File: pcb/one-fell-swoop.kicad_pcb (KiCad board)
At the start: 2 copper layers, 107.2 x 86.9 mm, 21 parts, among them J1 MJ-4PP-9, SW1 SW_PUSH, SW10 SW_PUSH, SW11 SW_PUSH, SW12 SW_PUSH, SW13 SW_PUSH, SW14 SW_PUSH, SW15 SW_PUSH, SW16 SW_PUSH, SW17 SW_PUSH, SW2 SW_PUSH, SW3 SW_PUSH, SW4 SW_PUSH, SW5 SW_PUSH, SW6 SW_PUSH, SW7 SW_PUSH, SW8 SW_PUSH, SW9 SW_PUSH, U1 ProMicro

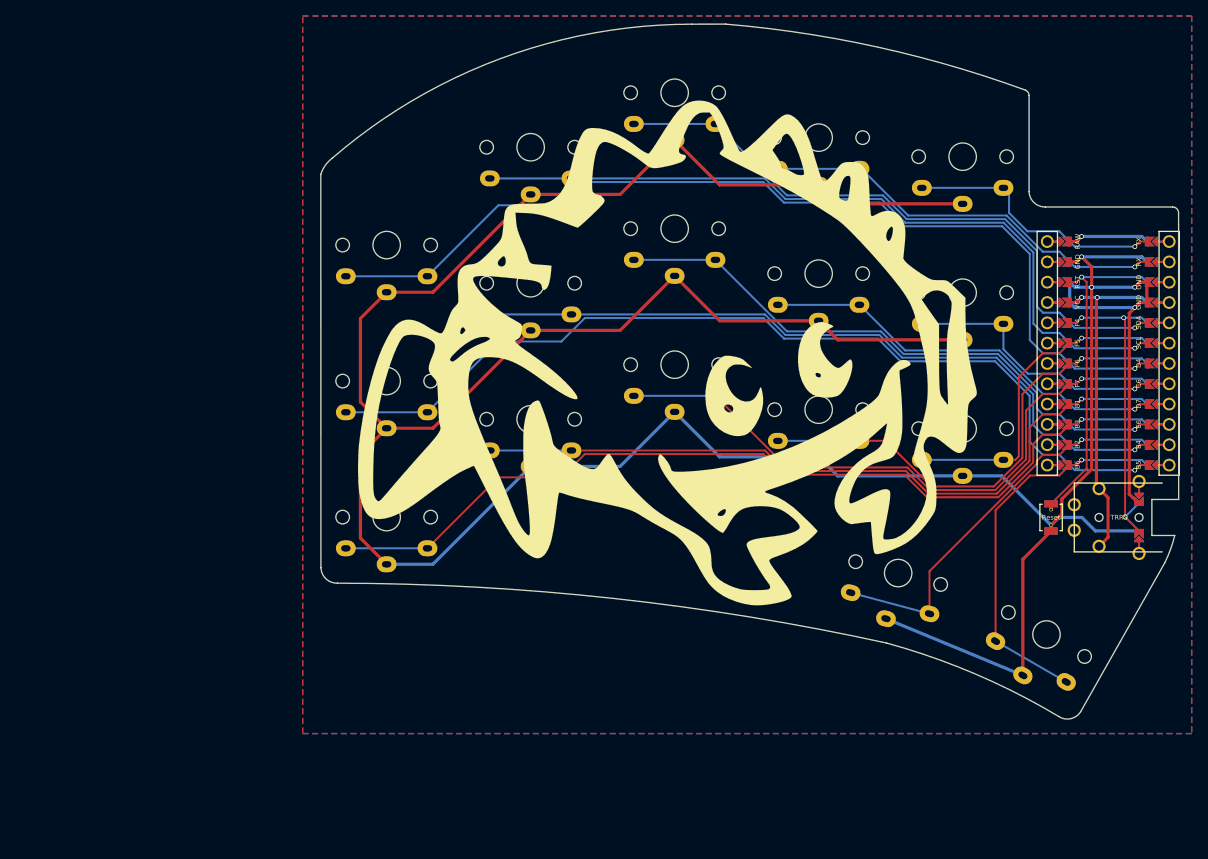
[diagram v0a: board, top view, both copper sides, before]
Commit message: Added files for the second version of the Swoop.
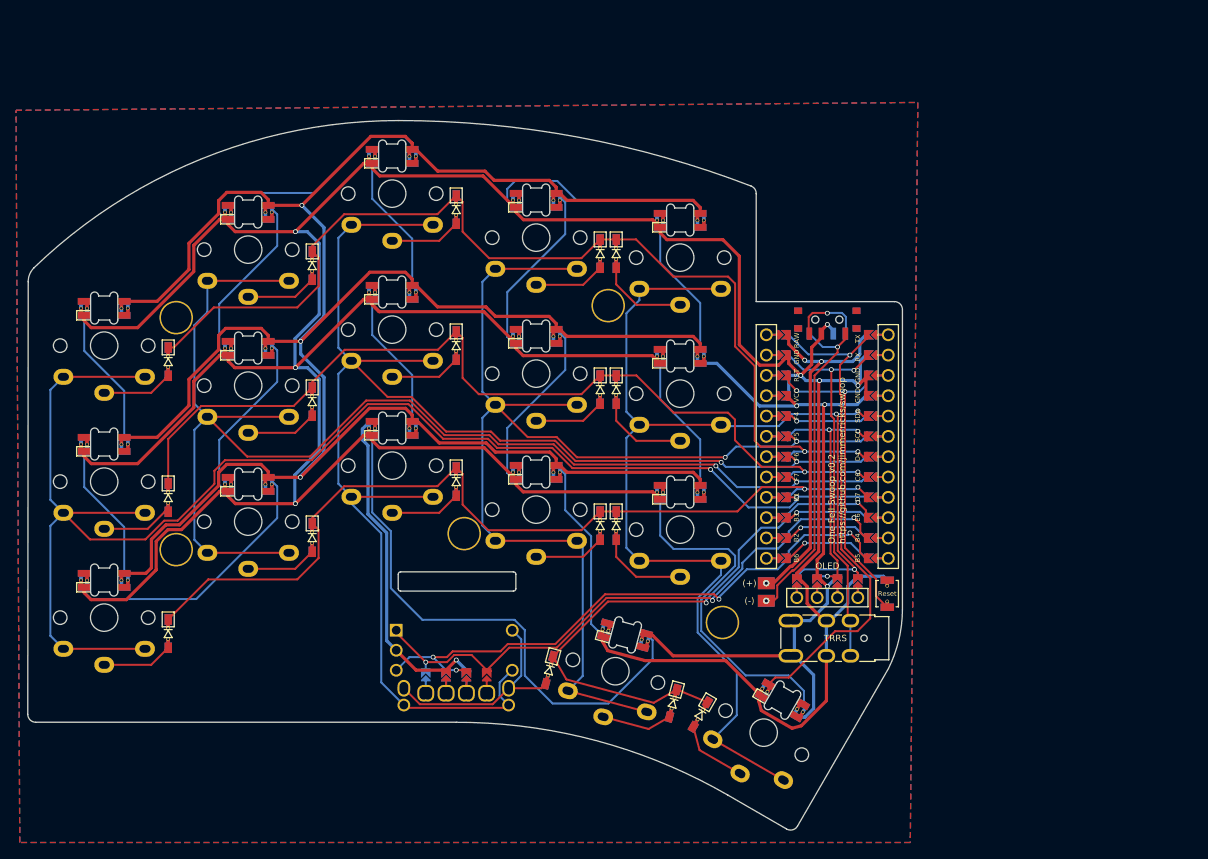
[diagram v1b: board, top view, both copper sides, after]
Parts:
- removed G***: LOGO, one-fell-swoop:Ferris_rust_logos
- added BT1: Battery, swoop:Battery_pads, F.Cu at (154.0, 118.0)
- added D1: 1N4148W, swoop:D3_SMD, F.Cu at (79.2, 89.2)
- added D10: 1N4148W, swoop:D3_SMD, F.Cu at (135.2, 92.7)
- added D11: 1N4148W, swoop:D3_SMD, F.Cu at (79.2, 123.2)
- added D12: 1N4148W, swoop:D3_SMD, F.Cu at (97.2, 111.2)
- added D13: 1N4148W, swoop:D3_SMD, F.Cu at (115.2, 104.2)
- added D14: 1N4148W, swoop:D3_SMD, F.Cu at (133.2, 109.7)
- added D15: 1N4148W, swoop:D3_SMD, F.Cu at (135.2, 109.7)
- added D16: 1N4148W, swoop:D3_SMD, F.Cu at (142.3, 131.9)
- added D17: 1N4148W, swoop:D3_SMD, F.Cu at (145.8, 133.4)
- added D2: 1N4148W, swoop:D3_SMD, F.Cu at (97.2, 77.2)
- added D3: 1N4148W, swoop:D3_SMD, F.Cu at (115.2, 70.2)
- added D4: 1N4148W, swoop:D3_SMD, F.Cu at (133.2, 75.7)
- added D5: 1N4148W, swoop:D3_SMD, F.Cu at (135.2, 75.7)
- added D6: 1N4148W, swoop:D3_SMD, F.Cu at (79.2, 106.2)
- added D7: 1N4148W, swoop:D3_SMD, F.Cu at (97.2, 94.2)
- added D8: 1N4148W, swoop:D3_SMD, F.Cu at (115.2, 87.2)
- added D9: 1N4148W, swoop:D3_SMD, F.Cu at (133.2, 92.7)
- added ED1: 1N4148W, swoop:D3_SMD, F.Cu at (126.9, 127.8)
- added EN1: RotaryEncoder_Switch, swoop:RotaryEncoder, F.Cu at (115.2, 125.3)
- added EN2: EVQWGD001, swoop:RollerEncoder, F.Cu at (115.2, 125.3)
- added H1: M2 Hole, swoop:M2_hole_4.2mm, F.Cu at (80.2, 83.7)
- added H2: M2 Hole, swoop:M2_hole_4.2mm, F.Cu at (80.2, 112.7)
- added H3: M2 Hole, swoop:M2_hole_4.2mm, F.Cu at (134.2, 82.2)
- added H4: M2 Hole, swoop:M2_hole_4.2mm, F.Cu at (116.2, 110.7)
- added H4: M2 Hole, swoop:M2_hole_4.2mm, F.Cu at (148.5, 121.9)
- added L1: SK6812Mini-e, swoop:SK6812_Mini_E, F.Cu at (71.2, 82.7)
- added L10: SK6812Mini-e, swoop:SK6812_Mini_E, F.Cu at (143.2, 88.7)
- added L11: SK6812Mini-e, swoop:SK6812_Mini_E, F.Cu at (71.2, 116.7)
- added L12: SK6812Mini-e, swoop:SK6812_Mini_E, F.Cu at (89.2, 104.7)
- added L13: SK6812Mini-e, swoop:SK6812_Mini_E, F.Cu at (107.2, 97.7)
- added L14: SK6812Mini-e, jmnw:sk6812_mini_e_rev, F.Cu at (125.2, 103.2)
- added L15: SK6812Mini-e, swoop:SK6812_Mini_E, F.Cu at (143.2, 105.7)
- added L16: SK6812Mini-e, swoop:SK6812_Mini_E, F.Cu at (136.3, 123.5)
- added L17: SK6812Mini-e, swoop:SK6812_Mini_E, F.Cu at (155.9, 131.7)
- added L2: SK6812Mini-e, swoop:SK6812_Mini_E, F.Cu at (89.2, 70.7)
- added L3: SK6812Mini-e, swoop:SK6812_Mini_E, F.Cu at (107.2, 63.7)
- added L4: SK6812Mini-e, swoop:SK6812_Mini_E, F.Cu at (125.2, 69.2)
- added L5: SK6812Mini-e, swoop:SK6812_Mini_E, F.Cu at (143.2, 71.7)
- added L6: SK6812Mini-e, swoop:SK6812_Mini_E, F.Cu at (71.2, 99.7)
- added L7: SK6812Mini-e, swoop:SK6812_Mini_E, F.Cu at (89.2, 87.7)
- added L8: SK6812Mini-e, swoop:SK6812_Mini_E, F.Cu at (107.2, 80.7)
- added L9: SK6812Mini-e, swoop:SK6812_Mini_E, F.Cu at (125.2, 86.2)
- added O1: OLED, swoop:OLED_jumpers, F.Cu at (157.8, 118.7)
- added PSW1: Power, jmnw:Power_reversible, F.Cu at (161.6, 84.0)
- J1: value MJ-4PP-9 -> TRRS; footprint one-fell-swoop:TRRS_jumpers -> swoop:TRRS-3pin
- RSW1: value SW_PUSH -> Reset; footprint one-fell-swoop:Reset_reversible -> swoop:Reset
- SW1, SW10, SW11, SW12, SW13, SW14, SW15, SW2, SW3, SW4, SW5, SW6, SW7, SW8, SW9: value SW_PUSH -> Choc; footprint one-fell-swoop:Choc_reversible -> swoop:Choc
- SW16, SW17: value SW_PUSH -> Choc; footprint one-fell-swoop:Choc_reversible -> swoop:Choc; moved to F.Cu
- U1: footprint one-fell-swoop:ProMicro_jumpers -> swoop:ProMicro_jumpers
- moved SW2 37.6 mm to (89.2, 75.2)
- moved SW7 37.6 mm to (89.2, 92.2)
- moved SW12 37.6 mm to (89.2, 109.2)
- moved SW10 37.5 mm to (143.2, 93.2)
- moved SW13 37.5 mm to (107.2, 102.2)
- moved SW8 37.5 mm to (107.2, 85.2)
- moved SW5 37.5 mm to (143.2, 76.2)
- moved SW15 37.5 mm to (143.2, 110.2)
- moved SW3 37.5 mm to (107.2, 68.2)
- moved SW1 37.5 mm to (71.2, 87.2)
- moved SW6 37.5 mm to (71.2, 104.2)
- moved SW11 37.5 mm to (71.2, 121.2)
- moved SW9 37.5 mm to (125.2, 90.7)
- moved SW4 37.5 mm to (125.2, 73.7)
- moved SW14 37.5 mm to (125.2, 107.7)
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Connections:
- J1 pad A: unconnected-(J1-PadA) -> VCC
- SW1 pad 1: switch1 -> col0
- SW1 pad 2: GND -> Net-(D1-Pad2)
- SW10 pad 1: switch10 -> col4
- SW10 pad 2: GND -> Net-(D10-Pad2)
- SW11 pad 1: switch11 -> col0
- SW11 pad 2: GND -> Net-(D11-Pad2)
- SW12 pad 1: switch12 -> col1
- SW12 pad 2: GND -> Net-(D12-Pad2)
- SW13 pad 1: switch13 -> col2
- SW13 pad 2: GND -> Net-(D13-Pad2)
- SW14 pad 1: switch14 -> col3
- SW14 pad 2: GND -> Net-(D14-Pad2)
- SW15 pad 1: switch15 -> col4
- SW15 pad 2: GND -> Net-(D15-Pad2)
- SW16 pad 1: switch16 -> col3
- SW16 pad 2: GND -> Net-(D16-Pad2)
- SW17 pad 1: switch17 -> col4
- SW17 pad 2: GND -> Net-(D17-Pad2)
- SW2 pad 1: switch2 -> col1
- SW2 pad 2: GND -> Net-(D2-Pad2)
- SW3 pad 1: switch3 -> col2
- SW3 pad 2: GND -> Net-(D3-Pad2)
- SW4 pad 1: switch4 -> col3
- SW4 pad 2: GND -> Net-(D4-Pad2)
- SW5 pad 1: switch5 -> col4
- SW5 pad 2: GND -> Net-(D5-Pad2)
- SW6 pad 1: switch6 -> col0
- SW6 pad 2: GND -> Net-(D6-Pad2)
- SW7 pad 1: switch7 -> col1
- SW7 pad 2: GND -> Net-(D7-Pad2)
- SW8 pad 1: switch8 -> col2
- SW8 pad 2: GND -> Net-(D8-Pad2)
- SW9 pad 1: switch9 -> col3
- SW9 pad 2: GND -> Net-(D9-Pad2)
- U1 pad 1: switch5 -> led
- U1 pad 10: switch8 -> row3
- U1 pad 11: switch7 -> eda
- U1 pad 12: switch6 -> edb
- U1 pad 13: switch17 -> unconnected-(U1-Pad13)
- U1 pad 14: switch16 -> unconnected-(U1-Pad14)
- U1 pad 15: switch11 -> unconnected-(U1-Pad15)
- U1 pad 16: switch12 -> col0
- U1 pad 17: switch13 -> col1
- U1 pad 18: switch14 -> col2
- U1 pad 19: switch15 -> col3
- U1 pad 2: switch4 -> data
- U1 pad 20: data -> col4
- U1 pad 24: unconnected-(U1-Pad24) -> raw
- U1 pad 5: switch3 -> sda
- U1 pad 6: switch2 -> sla
- U1 pad 7: switch1 -> row0
- U1 pad 8: switch10 -> row1
- U1 pad 9: switch9 -> row2
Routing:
- net VCC: track 42.4 -> 402.0 mm, vias 2 -> 6
- net col2: track 0.00 -> 186.5 mm, vias 0 -> 2
- net col0: track 0.00 -> 184.1 mm, vias 0 -> 2
- net col1: track 0.00 -> 160.8 mm, vias 0 -> 2
- net col3: track 0.00 -> 148.7 mm, vias 0 -> 2
- net row0: track 0.00 -> 129.1 mm, vias 0 -> 2
- net col4: track 0.00 -> 123.5 mm, vias 0 -> 1
- net switch1: track 121.2 -> 0.00 mm, vias 1 -> 0
- net switch6: track 116.5 -> 0.00 mm, vias 1 -> 0
- net row1: track 0.00 -> 114.9 mm, vias 0 -> 2
- net switch11: track 112.9 -> 0.00 mm, vias 1 -> 0
- net row2: track 0.00 -> 110.2 mm, vias 0 -> 2
- net switch2: track 96.4 -> 0.00 mm, vias 1 -> 0
- net switch12: track 92.0 -> 0.00 mm, vias 1 -> 0
- net switch7: track 91.6 -> 0.00 mm, vias 1 -> 0
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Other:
- board size 107.2 x 86.9 mm -> 109.3 x 88.7 mm
- board text added: "One Fell Swoop v0.2 https://github.com/jimmerricks/swoop"
